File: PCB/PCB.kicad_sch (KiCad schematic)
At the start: 51 parts, among them J1 USB_C_Receptacle_USB2.0_16P, Q1 NMOS, SW1 RESET, SW2 Button, U1 RP2040, U2 W25Q32JVSS, U4 NCP1117-3.3_SOT223, Y1 12 MHz

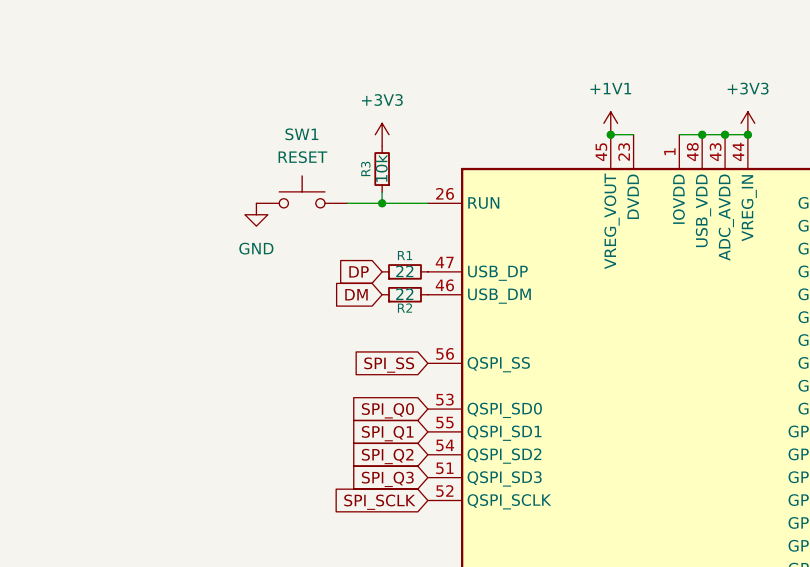
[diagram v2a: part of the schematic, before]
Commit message: potato
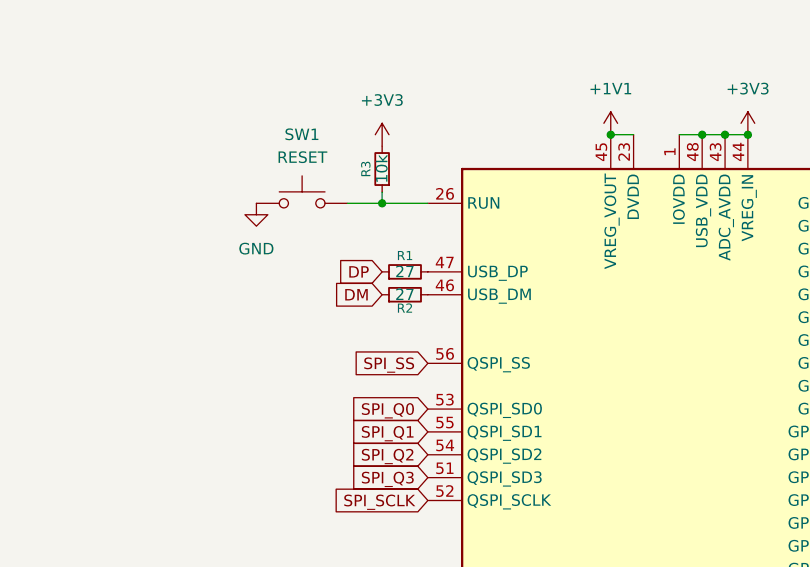
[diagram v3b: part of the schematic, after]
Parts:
- C1, C10, C11, C12, C13, C14, C15, C16, C17, C18, C19, C2, C20, C21, C22, C23, C24, C25, C26, C3, C4, C5, C6, C7, C8, C9: footprint Capacitor_SMD:C_01005_0402Metric -> Capacitor_SMD:C_0402_1005Metric
- R1, R2: value 22 -> 27; footprint Resistor_SMD:R_01005_0402Metric -> Resistor_SMD:R_0402_1005Metric
- R10, R11, R3, R4, R5, R6, R7, R8, R9: footprint Resistor_SMD:R_01005_0402Metric -> Resistor_SMD:R_0402_1005Metric
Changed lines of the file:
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@@
 			)
 		)
-		(property "Footprint" "Capacitor_SMD:C_01005_0402Metric"
+		(property "Footprint" "Capacitor_SMD:C_0402_1005Metric"
 			(at 544.83 49.53 0)
 			(effects
@@
 			)
 		)
-		(property "Footprint" "Capacitor_SMD:C_01005_0402Metric"
+		(property "Footprint" "Capacitor_SMD:C_0402_1005Metric"
 			(at 340.36 231.14 0)
 			(effects
@@
 			)
 		)
-		(property "Footprint" "Capacitor_SMD:C_01005_0402Metric"
+		(property "Footprint" "Capacitor_SMD:C_0402_1005Metric"
 			(at 520.7 49.53 0)
 			(effects
@@
 			)
 		)
-		(property "Footprint" "Capacitor_SMD:C_01005_0402Metric"
+		(property "Footprint" "Capacitor_SMD:C_0402_1005Metric"
 			(at 332.74 248.92 0)
 			(effects
@@
 			)
 		)
-		(property "Footprint" "Capacitor_SMD:C_01005_0402Metric"
+		(property "Footprint" "Capacitor_SMD:C_0402_1005Metric"
 			(at 336.55 251.46 0)
 			(effects
@@
 			)
 		)
-		(property "Footprint" "Capacitor_SMD:C_01005_0402Metric"
+		(property "Footprint" "Capacitor_SMD:C_0402_1005Metric"
 			(at 387.35 232.41 0)
 			(effects
@@
 			)
 		)
-		(property "Footprint" "Resistor_SMD:R_01005_0402Metric"
+		(property "Footprint" "Resistor_SMD:R_0402_1005Metric"
 			(at 528.32 168.91 0)
 			(effects
@@
 			)
 		)
-		(property "Footprint" "Resistor_SMD:R_01005_0402Metric"
+		(property "Footprint" "Resistor_SMD:R_0402_1005Metric"
 			(at 347.98 59.69 0)
 			(effects
@@
 			)
 		)
-		(property "Footprint" "Resistor_SMD:R_01005_0402Metric"
+		(property "Footprint" "Resistor_SMD:R_0402_1005Metric"
 			(at 425.45 80.01 0)
 			(effects
@@
 			)
 		)
-		(property "Footprint" "Capacitor_SMD:C_01005_0402Metric"
+		(property "Footprint" "Capacitor_SMD:C_0402_1005Metric"
 			(at 353.06 243.84 0)
 			(effects
@@
 			)
 		)
-		(property "Footprint" "Resistor_SMD:R_01005_0402Metric"
+		(property "Footprint" "Resistor_SMD:R_0402_1005Metric"
 			(at 360.68 166.37 0)
 			(effects
@@
 			)
 		)
-		(property "Footprint" "Resistor_SMD:R_01005_0402Metric"
+		(property "Footprint" "Resistor_SMD:R_0402_1005Metric"
 			(at 347.98 57.15 0)
 			(effects
@@
 			)
 		)
-		(property "Footprint" "Capacitor_SMD:C_01005_0402Metric"
+		(property "Footprint" "Capacitor_SMD:C_0402_1005Metric"
 			(at 335.28 236.22 0)
 			(effects
@@
 			)
 		)
-		(property "Footprint" "Capacitor_SMD:C_01005_0402Metric"
+		(property "Footprint" "Capacitor_SMD:C_0402_1005Metric"
 			(at 386.08 52.07 0)
 			(effects
@@
 			)
 		)
-		(property "Footprint" "Capacitor_SMD:C_01005_0402Metric"
+		(property "Footprint" "Capacitor_SMD:C_0402_1005Metric"
 			(at 466.09 49.53 0)
 			(effects
@@
 			)
 		)
-		(property "Footprint" "Capacitor_SMD:C_01005_0402Metric"
+		(property "Footprint" "Capacitor_SMD:C_0402_1005Metric"
 			(at 433.07 49.53 0)
 			(effects
@@
 			)
 		)
-		(property "Footprint" "Capacitor_SMD:C_01005_0402Metric"
+		(property "Footprint" "Capacitor_SMD:C_0402_1005Metric"
 			(at 548.64 161.29 0)
 			(effects
@@
 			)
 		)
-		(property "Footprint" "Capacitor_SMD:C_01005_0402Metric"
+		(property "Footprint" "Capacitor_SMD:C_0402_1005Metric"
 			(at 477.52 49.53 0)
 			(effects
@@
 			)
 		)
-		(property "Footprint" "Capacitor_SMD:C_01005_0402Metric"
+		(property "Footprint" "Capacitor_SMD:C_0402_1005Metric"
 			(at 497.84 49.53 0)
 			(effects
@@
 			)
 		)
-		(property "Footprint" "Capacitor_SMD:C_01005_0402Metric"
+		(property "Footprint" "Capacitor_SMD:C_0402_1005Metric"
 			(at 533.4 49.53 0)
 			(effects
@@
 			)
 		)
-		(property "Footprint" "Capacitor_SMD:C_01005_0402Metric"
+		(property "Footprint" "Capacitor_SMD:C_0402_1005Metric"
 			(at 443.23 49.53 0)
 			(effects
@@
 			)
 		)
-		(property "Footprint" "Resistor_SMD:R_01005_0402Metric"
+		(property "Footprint" "Resistor_SMD:R_0402_1005Metric"
 			(at 387.35 264.16 0)
 			(effects
@@
 			)
 		)
-		(property "Footprint" "Capacitor_SMD:C_01005_0402Metric"
+		(property "Footprint" "Capacitor_SMD:C_0402_1005Metric"
 			(at 337.82 166.37 0)
 			(effects
@@
 			)
 		)
-		(property "Footprint" "Capacitor_SMD:C_01005_0402Metric"
+		(property "Footprint" "Capacitor_SMD:C_0402_1005Metric"
 			(at 487.68 49.53 0)
 			(effects
@@
 			)
 		)
-		(property "Footprint" "Capacitor_SMD:C_01005_0402Metric"
+		(property "Footprint" "Capacitor_SMD:C_0402_1005Metric"
 			(at 368.3 247.65 0)
 			(effects
@@
 			)
 		)
-		(property "Footprint" "Capacitor_SMD:C_01005_0402Metric"
+		(property "Footprint" "Capacitor_SMD:C_0402_1005Metric"
 			(at 421.64 49.53 0)
 			(effects
@@
 			)
 		)
-		(property "Footprint" "Resistor_SMD:R_01005_0402Metric"
+		(property "Footprint" "Resistor_SMD:R_0402_1005Metric"
 			(at 369.57 96.52 0)
 			(effects
@@
 			)
 		)
-		(property "Footprint" "Resistor_SMD:R_01005_0402Metric"
+		(property "Footprint" "Resistor_SMD:R_0402_1005Metric"
 			(at 379.73 264.16 0)
 			(effects
@@
 			)
 		)
-		(property "Footprint" "Capacitor_SMD:C_01005_0402Metric"
+		(property "Footprint" "Capacitor_SMD:C_0402_1005Metric"
 			(at 346.71 241.3 0)
 			(effects
@@
 			)
 		)
-		(property "Value" "22"
+		(property "Value" "27"
 			(at 427.99 93.98 90)
 			(effects
@@
 			)
 		)
-		(property "Footprint" "Resistor_SMD:R_01005_0402Metric"
+		(property "Footprint" "Resistor_SMD:R_0402_1005Metric"
 			(at 427.99 93.98 0)
 			(effects
@@
 			)
 		)
-		(property "Value" "22"
+		(property "Value" "27"
 			(at 427.99 91.44 90)
 			(effects
@@
 			)
 		)
-		(property "Footprint" "Resistor_SMD:R_01005_0402Metric"
+		(property "Footprint" "Resistor_SMD:R_0402_1005Metric"
 			(at 427.99 91.44 0)
 			(effects
@@
 			)
 		)
-		(property "Footprint" "Capacitor_SMD:C_01005_0402Metric"
+		(property "Footprint" "Capacitor_SMD:C_0402_1005Metric"
 			(at 337.82 158.75 0)
 			(effects
@@
 			)
 		)
-		(property "Footprint" "Capacitor_SMD:C_01005_0402Metric"
+		(property "Footprint" "Capacitor_SMD:C_0402_1005Metric"
 			(at 341.63 246.38 0)
 			(effects
@@
 			)
 		)
-		(property "Footprint" "Capacitor_SMD:C_01005_0402Metric"
+		(property "Footprint" "Capacitor_SMD:C_0402_1005Metric"
 			(at 509.27 49.53 0)
 			(effects
@@
 			)
 		)
-		(property "Footprint" "Capacitor_SMD:C_01005_0402Metric"
+		(property "Footprint" "Capacitor_SMD:C_0402_1005Metric"
 			(at 336.55 203.2 0)
 			(effects
@@
 			)
 		)
-		(property "Footprint" "Capacitor_SMD:C_01005_0402Metric"
+		(property "Footprint" "Capacitor_SMD:C_0402_1005Metric"
 			(at 363.22 52.07 0)
 			(effects
@@
 			)
 		)
-		(property "Footprint" "Resistor_SMD:R_01005_0402Metric"
+		(property "Footprint" "Resistor_SMD:R_0402_1005Metric"
 			(at 520.7 171.45 0)
 			(effects

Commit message: commit
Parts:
- C21, C23: footprint Capacitor_SMD:C_0402_1005Metric -> Capacitor_SMD:C_0603_1608Metric
- C22, C24: footprint Capacitor_SMD:C_0402_1005Metric -> Capacitor_SMD:C_0805_2012Metric
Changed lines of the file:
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@@
 			)
 		)
-		(property "Footprint" "Capacitor_SMD:C_0402_1005Metric"
+		(property "Footprint" "Capacitor_SMD:C_0603_1608Metric"
 			(at 387.35 232.41 0)
 			(effects
@@
 			)
 		)
-		(property "Footprint" "Capacitor_SMD:C_0402_1005Metric"
+		(property "Footprint" "Capacitor_SMD:C_0805_2012Metric"
 			(at 386.08 52.07 0)
 			(effects
@@
 			)
 		)
-		(property "Footprint" "Capacitor_SMD:C_0402_1005Metric"
+		(property "Footprint" "Capacitor_SMD:C_0603_1608Metric"
 			(at 368.3 247.65 0)
 			(effects
@@
 			)
 		)
-		(property "Footprint" "Capacitor_SMD:C_0402_1005Metric"
+		(property "Footprint" "Capacitor_SMD:C_0805_2012Metric"
 			(at 363.22 52.07 0)
 			(effects

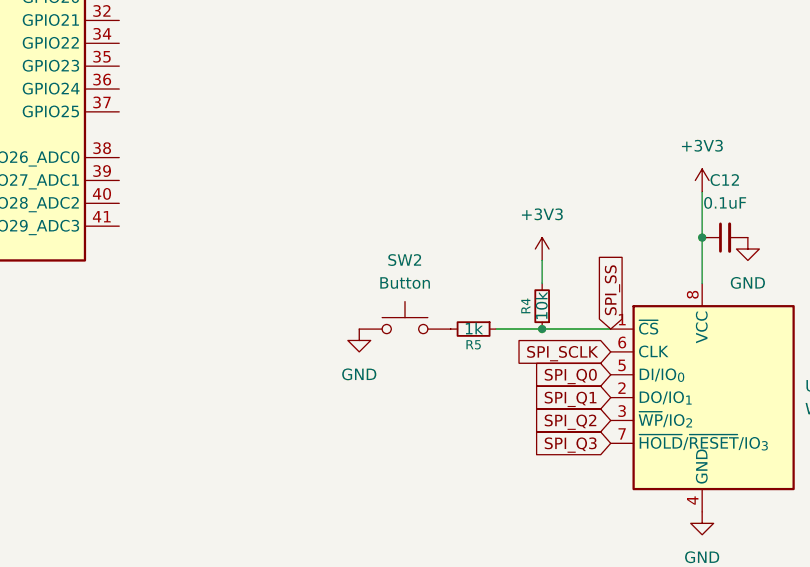
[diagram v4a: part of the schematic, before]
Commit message: COMMIT
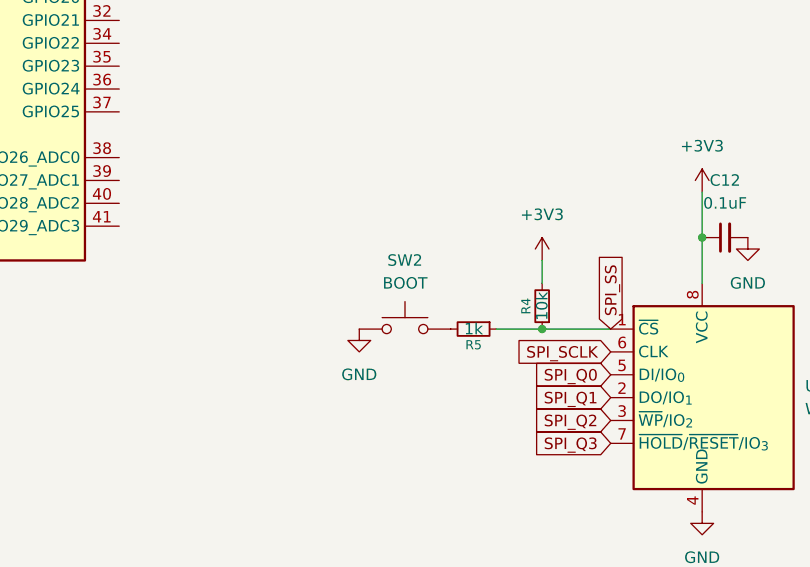
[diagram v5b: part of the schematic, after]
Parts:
- SW2: value Button -> BOOT
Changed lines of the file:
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@@
 			)
 		)
-		(property "Value" "Button"
+		(property "Value" "BOOT"
 			(at 513.08 166.37 0)
 			(effects
